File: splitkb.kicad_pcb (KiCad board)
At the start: 2 copper layers, 153 x 121.3 mm, 80 parts, among them J1 MJ-4PP-9, K1 KEYSW, SW1 SW_PUSH, SW10 SW_PUSH, SW11 SW_PUSH, SW12 SW_PUSH, SW13 SW_PUSH, SW14 SW_PUSH, SW15 SW_PUSH, SW16 SW_PUSH, SW17 SW_PUSH, SW18 SW_PUSH, SW19 SW_PUSH, SW2 SW_PUSH, SW20 SW_PUSH, SW21 SW_PUSH, SW22 SW_PUSH, SW23 SW_PUSH, SW24 SW_PUSH, SW25 SW_PUSH, SW26 SW_PUSH, SW27 SW_PUSH, SW28 SW_PUSH, SW29 SW_PUSH, SW3 SW_PUSH, SW30 SW_PUSH, SW31 SW_PUSH, SW32 SW_PUSH, SW4 SW_PUSH, SW5 SW_PUSH, SW6 SW_PUSH, SW7 SW_PUSH, SW8 SW_PUSH, SW9 SW_PUSH, U1 ProMicro

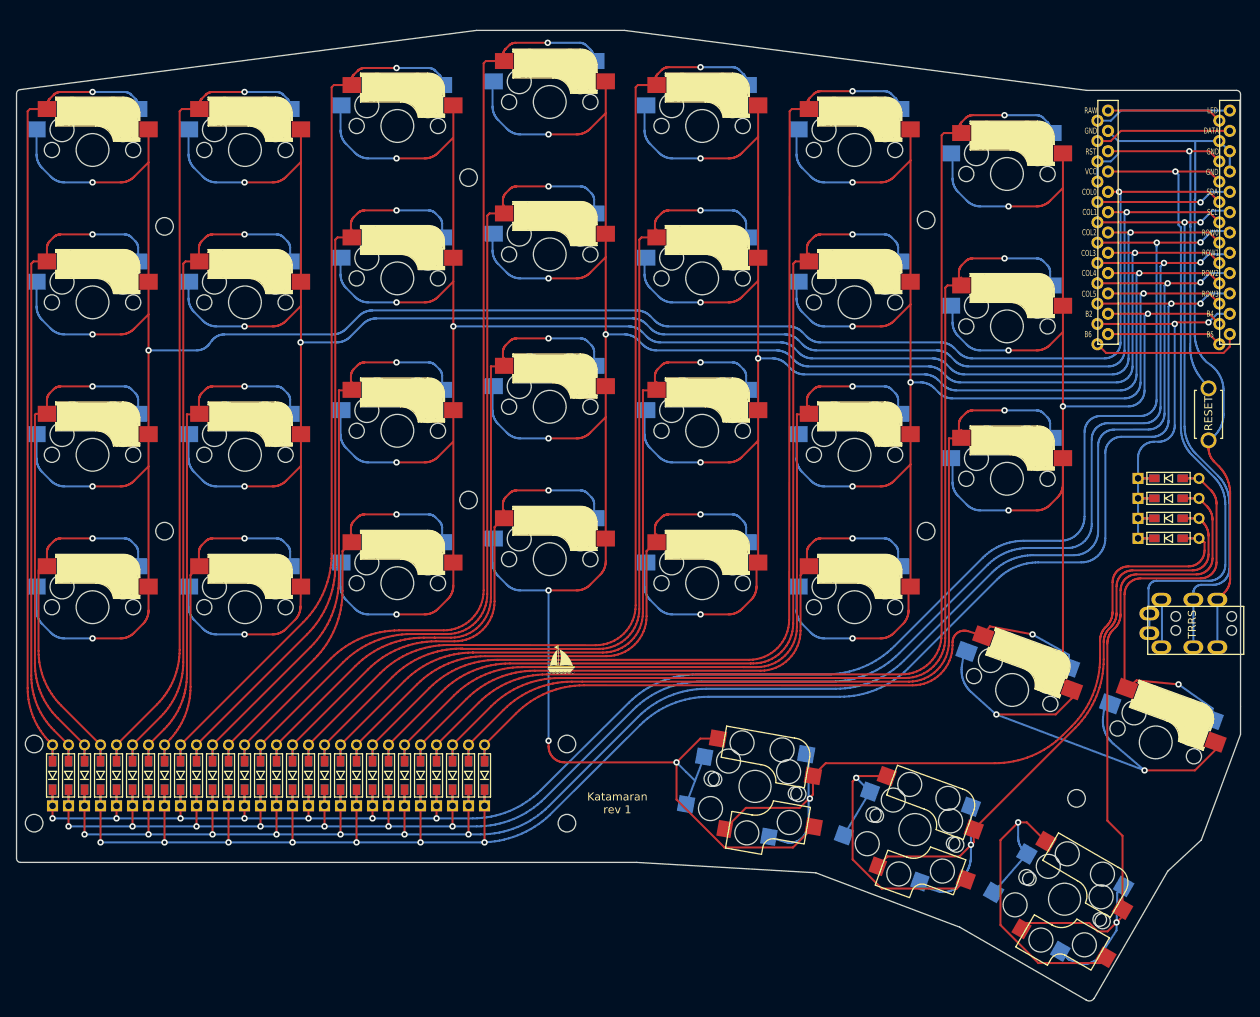
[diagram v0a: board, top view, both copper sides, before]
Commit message: waves
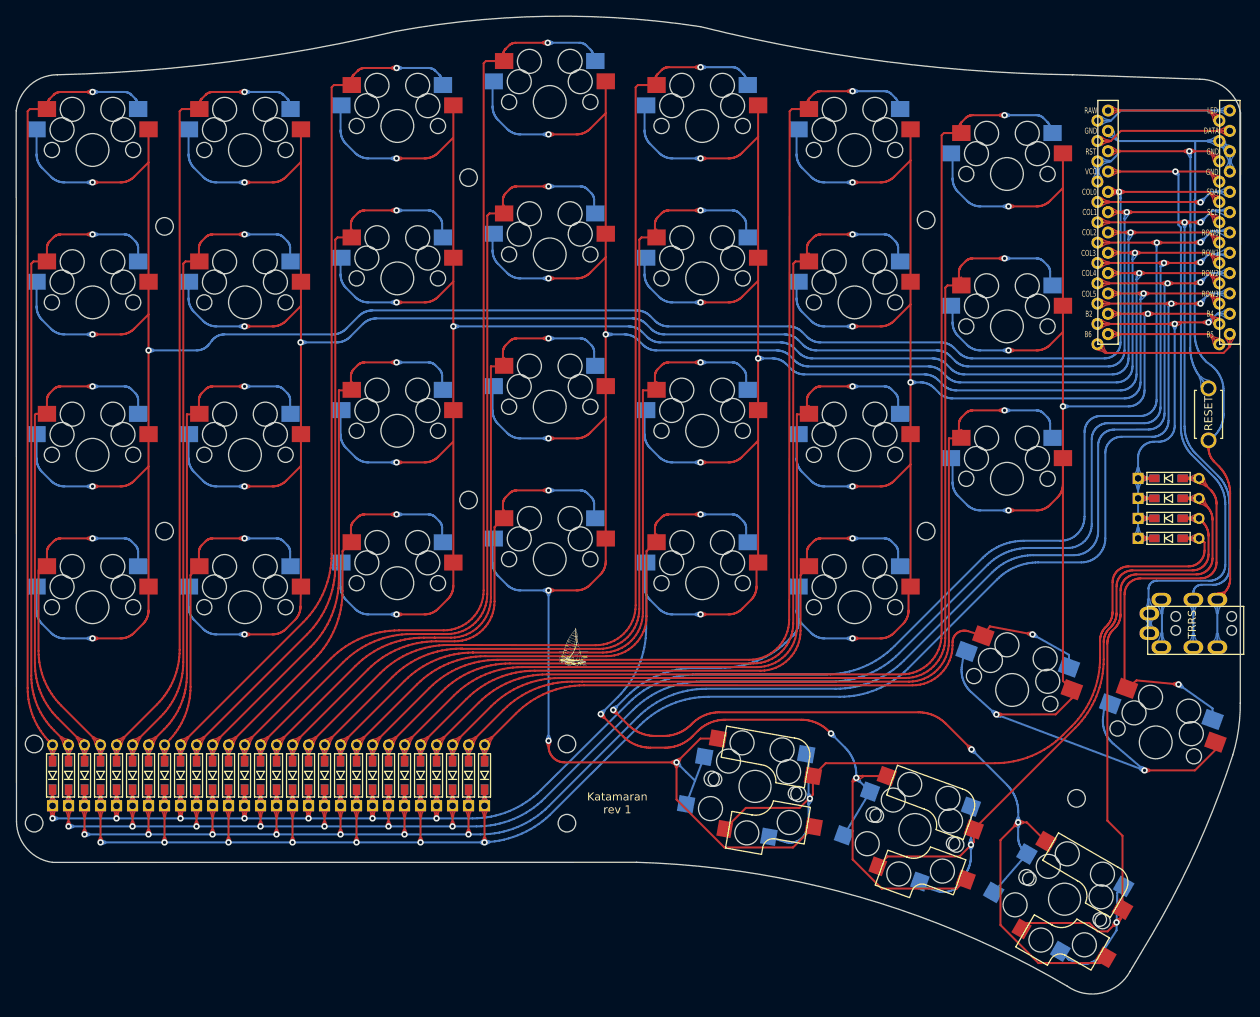
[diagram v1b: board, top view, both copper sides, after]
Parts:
- removed the   at (106.6, 113.7)
- removed G***: LOGO, picture:boat
- added  : LOGO, picture:katamaran, F.Cu at (108.1, 112.1)
- added  : LOGO, picture:katamaran, B.Cu at (162.6, 98.9)
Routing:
- net col5: track 241.3 -> 332.7 mm, vias 7 -> 9
- net col4: track 256.9 -> 316.2 mm, vias 7 -> 9
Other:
- board size 153 x 121.3 mm -> 153 x 122.2 mm
